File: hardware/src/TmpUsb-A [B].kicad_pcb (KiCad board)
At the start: 2 copper layers, 25 x 17 mm, 17 parts, among them P1 48037-2200, U1 PIC18F26J50

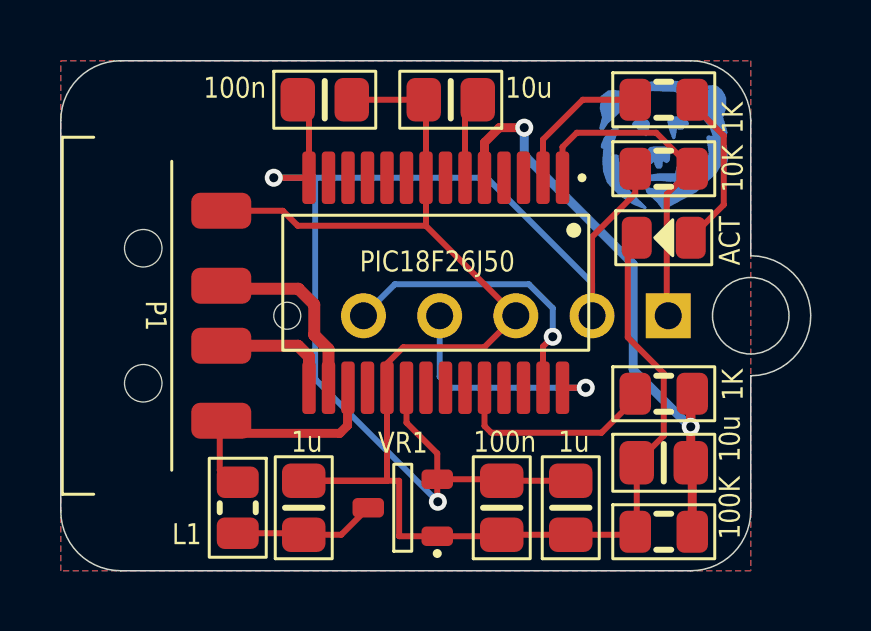
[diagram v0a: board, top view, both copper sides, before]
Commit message: Added schematics
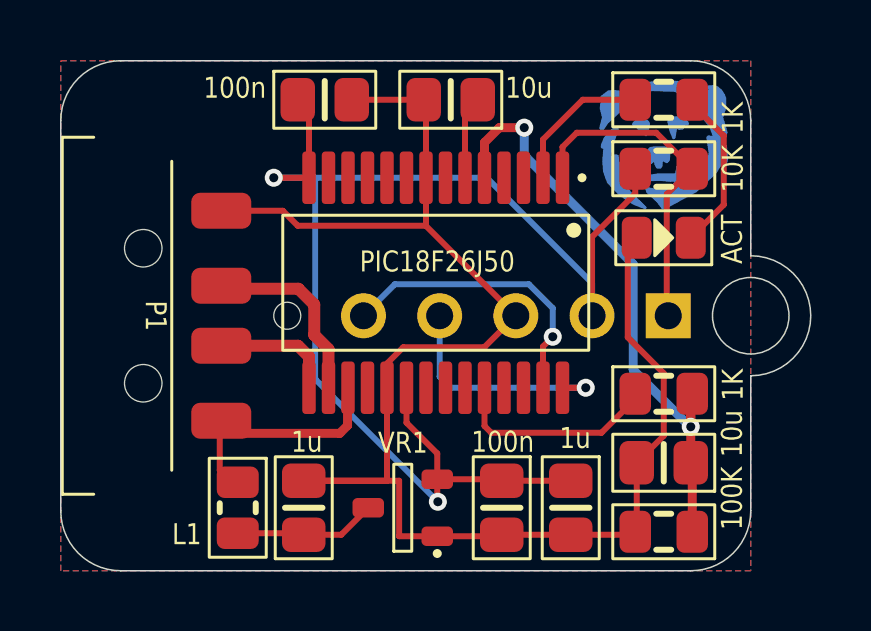
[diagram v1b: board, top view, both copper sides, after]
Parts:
- turned C1 to -90 degrees
- turned C4 to -90 degrees
- turned C6 to 180 degrees
- turned DS1 to 180 degrees
- turned R4 to 180 degrees
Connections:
- net 5V renamed +5V
- net USB_5V renamed VCC
- ? pad 2: 3V3 -> +3.3V
- C1 pad 1: GND -> +3.3V
- C1 pad 2: 3V3 -> GND
- C2 pad 1: 3V3 -> +3.3V
- C4 pad 1: GND -> +3.3V
- C4 pad 2: 3V3 -> GND
- C6 pad 1: GND -> CAP
- C6 pad 2: CAP -> GND
- DS1 pad 1: (no net) -> LED'
- DS1 pad 2: (no net) -> GND
- R3 pad 1: 3V3 -> +3.3V
- R4 pad 1: GND -> CAP
- R4 pad 2: CAP -> GND
- U1 pad 14: 3V3 -> +3.3V
- U1 pad 20: 3V3 -> +3.3V
- VR1 pad 2: 3V3 -> +3.3V
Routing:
- net 3V3: track 44.2 -> 0.00 mm, vias 2 -> 0
- net +3.3V: track 0.00 -> 44.2 mm, vias 0 -> 2
